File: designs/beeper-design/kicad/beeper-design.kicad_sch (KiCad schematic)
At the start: 0 parts

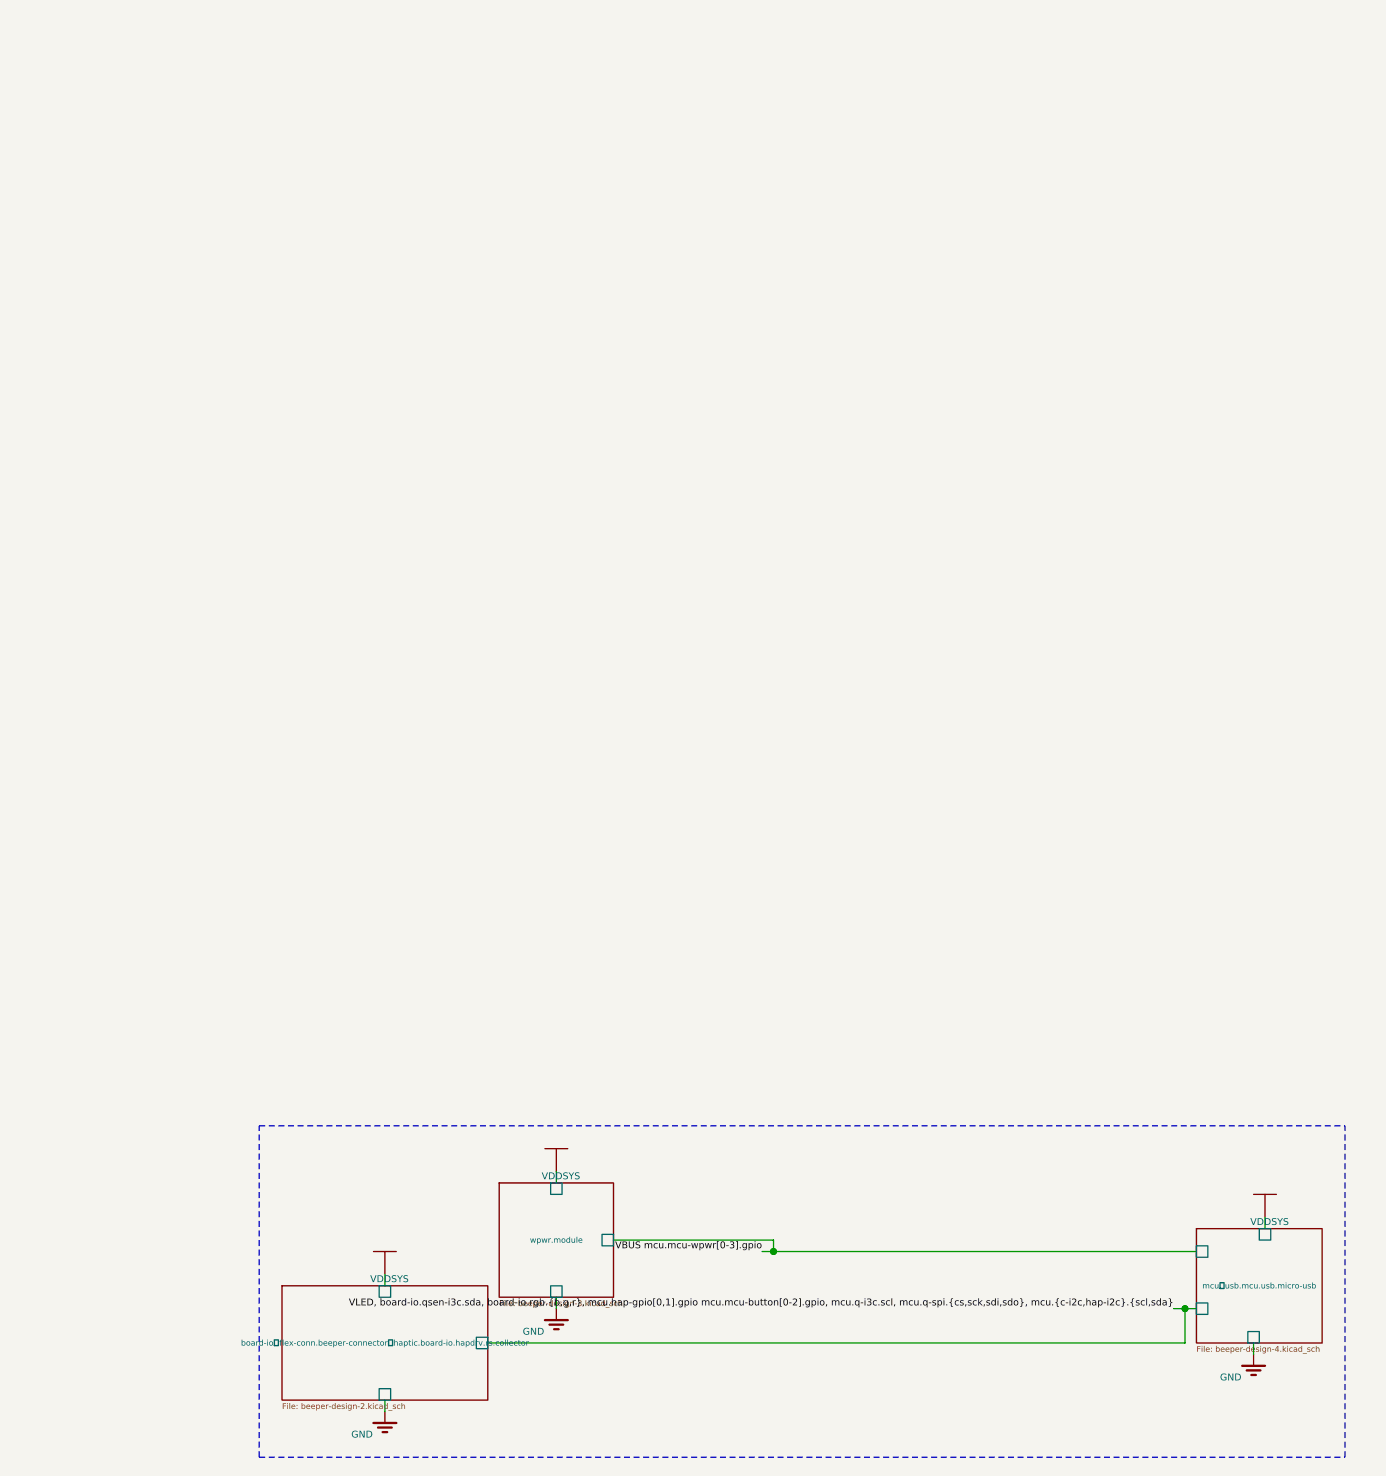
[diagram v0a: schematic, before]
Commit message: post export, had to munge sch
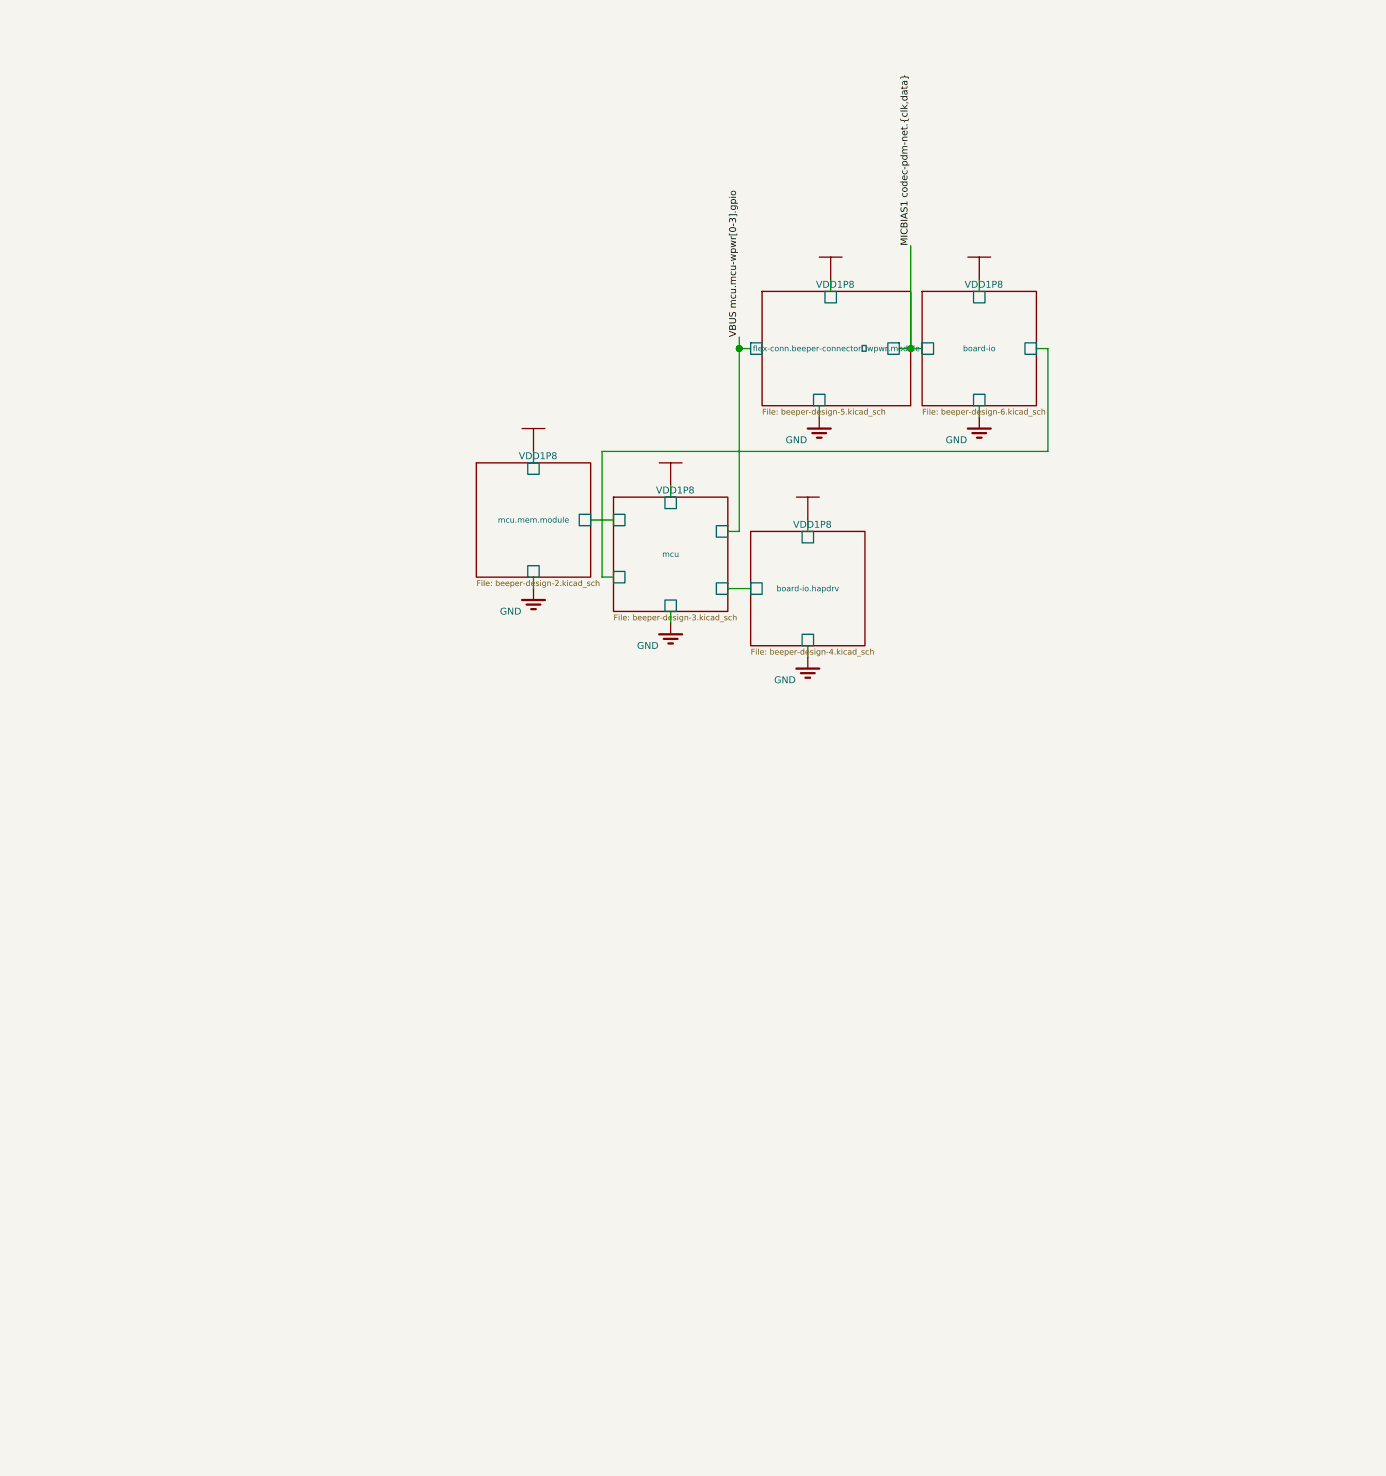
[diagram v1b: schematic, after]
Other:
- removed sheet board-io flex-conn.beeper-connector haptic.board-io.hapdrv.rs.collector
- removed sheet mcu usb.mcu.usb.micro-usb
- removed sheet wpwr.module
- added sheet board-io (beeper-design-6.kicad_sch)
- added sheet board-io.hapdrv (beeper-design-4.kicad_sch)
- added sheet flex-conn.beeper-connector wpwr.module (beeper-design-5.kicad_sch)
- added sheet mcu (beeper-design-3.kicad_sch)
- added sheet mcu.mem.module (beeper-design-2.kicad_sch)
